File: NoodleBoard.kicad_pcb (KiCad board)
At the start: 2 copper layers, 21 x 51.1 mm, 37 parts, among them J1 USB_C_Receptacle_USB2.0_16P, J2 Left, J3 Right, J4 Middle, J5 Bottom, SW1 Boot, SW2 Reset, U1 RP2040, U2 ME6211C33M5, U3 W25Q16JVZPIQ TR, Y1 12MHz

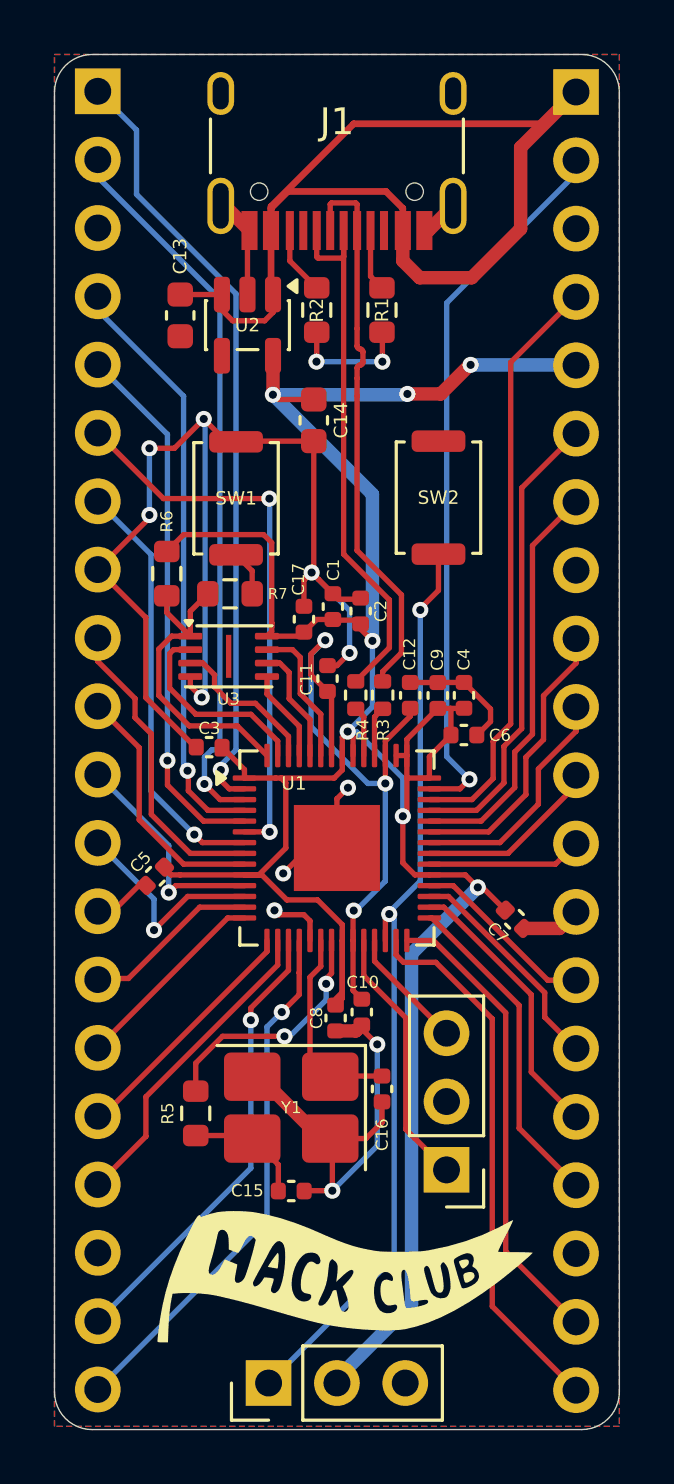
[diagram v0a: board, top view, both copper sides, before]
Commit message: feat: add all the files
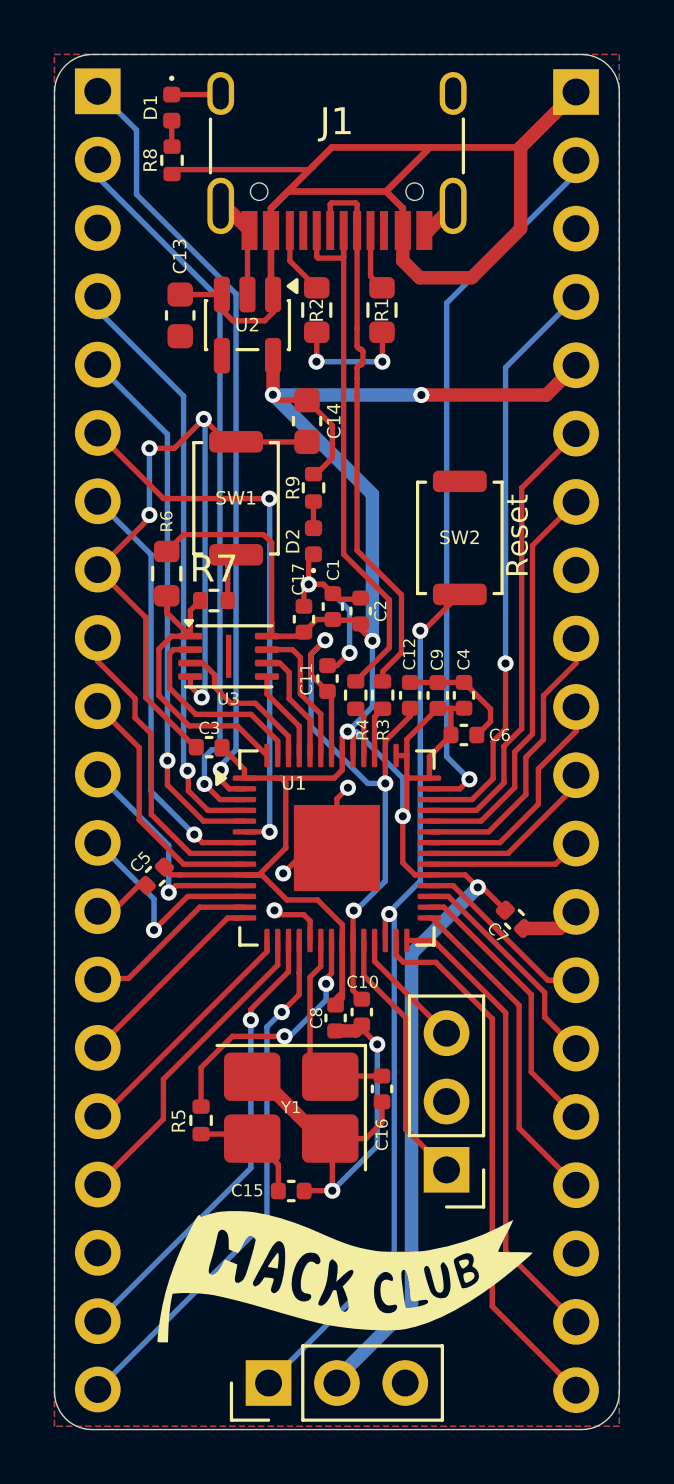
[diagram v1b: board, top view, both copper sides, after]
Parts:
- added D1: LED, LED_SMD:LED_0402_1005Metric, F.Cu at (18.4, 16.0)
- added D2: LED, LED_SMD:LED_0402_1005Metric, F.Cu at (23.6, 32.1)
- added R8: 1k, Resistor_SMD:R_0402_1005Metric, F.Cu at (18.4, 17.9)
- added R9: 1k, Resistor_SMD:R_0402_1005Metric, F.Cu at (23.6, 30.1)
- R5: value 5.1k -> 1k; footprint Resistor_SMD:R_0603_1608Metric -> Resistor_SMD:R_0402_1005Metric
- R7: footprint Resistor_SMD:R_0603_1608Metric -> Resistor_SMD:R_0402_1005Metric
- moved SW2 1.69 mm to (29.1, 32.0)
- moved R7 0.65 mm to (19.9, 34.3)
- moved R5 0.33 mm to (19.4, 53.6)
- moved C14 0.25 mm to (23.4, 27.6)
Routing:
- net VBUS: track 40.9 -> 44.8 mm
- net +3V3: track 108.8 -> 112.3 mm, vias 7 -> 6
- net GND: track 88.8 -> 86.1 mm
- net /RUN: track 34.6 -> 33.5 mm
- net Net-(D2-A): track 0.00 -> 0.99 mm
- net Net-(D1-A): track 0.00 -> 0.97 mm
- net /GPIO28_ADC2: vias 0 -> 1
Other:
- board text added: "Reset"

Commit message: make pcb a bit better
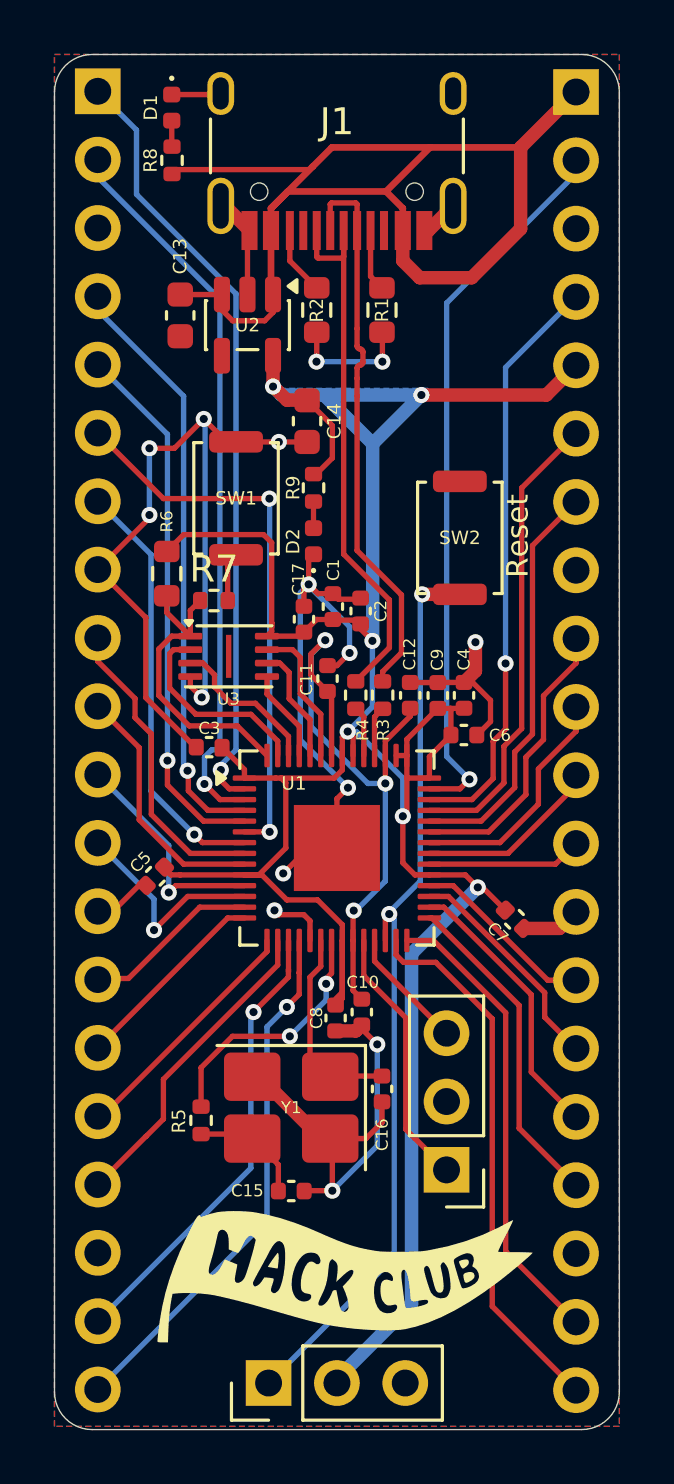
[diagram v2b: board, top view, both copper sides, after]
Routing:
- net GND: track 86.1 -> 96.2 mm, vias 13 -> 15
- net +3V3: track 112.3 -> 114.0 mm
- net /RUN: track 33.5 -> 34.3 mm
- added copper zone on B.Cu, net +3V3
